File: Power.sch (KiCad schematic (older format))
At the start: 82 parts, among them J3 USB, J4 OTG, Q1 DTA114YKA, SW1 PWRON, SW2 RST, U1 AllWinner-S3(FBGA-234), U3 AXP209(QFN-48), U4 SY8089AAAC, U5 SY6280AAC

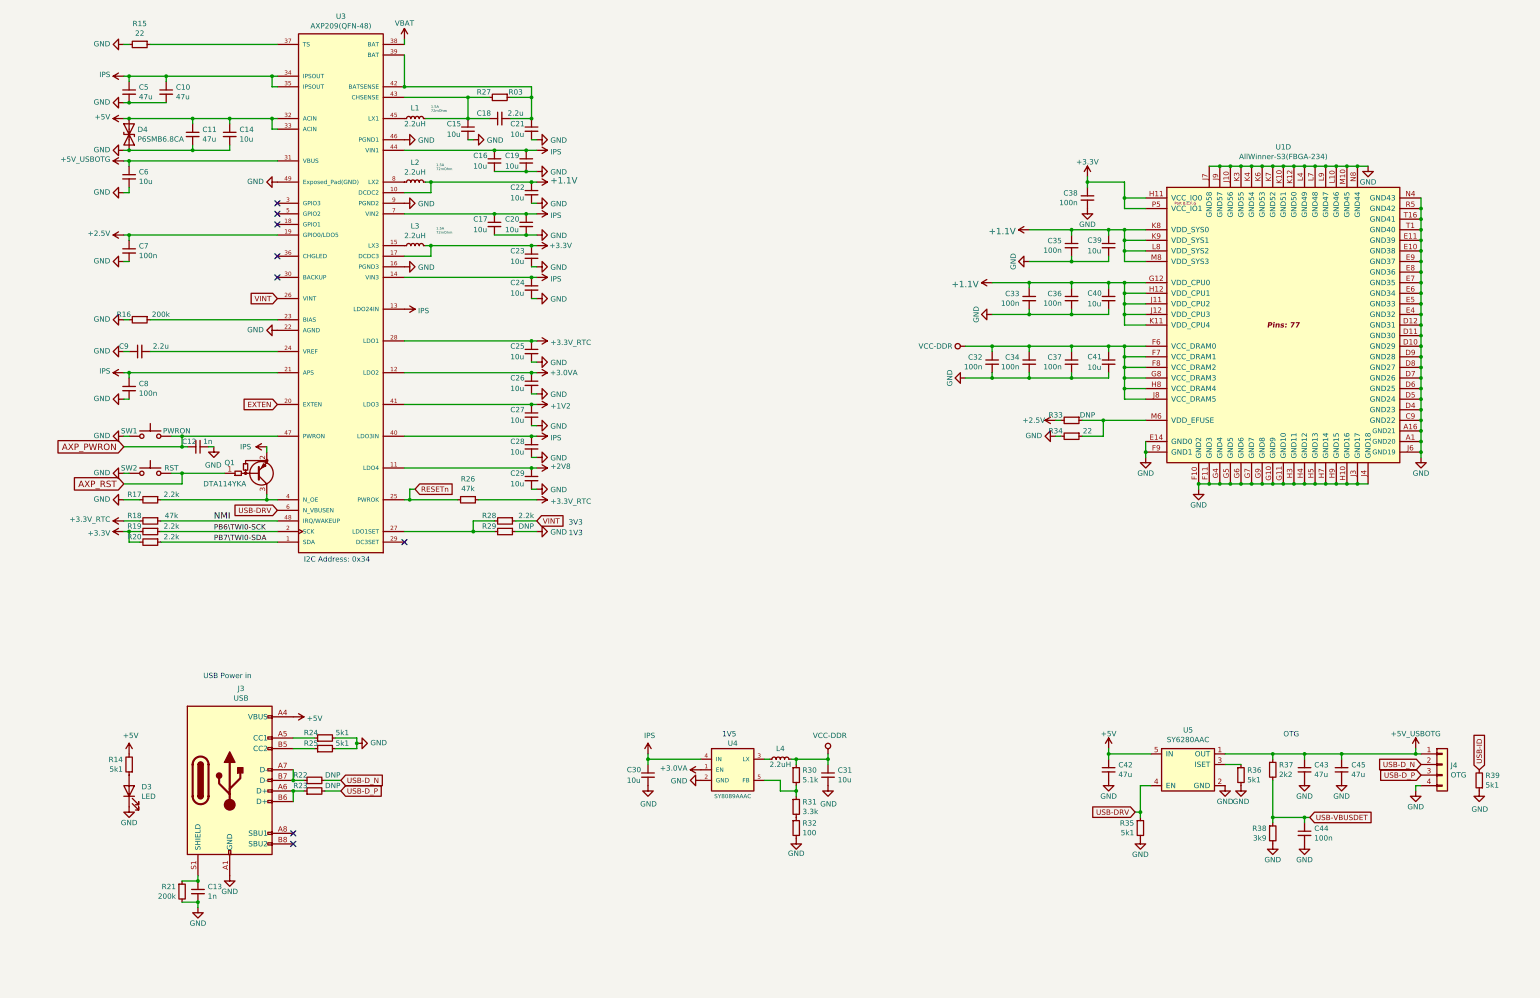
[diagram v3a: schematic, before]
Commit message: update
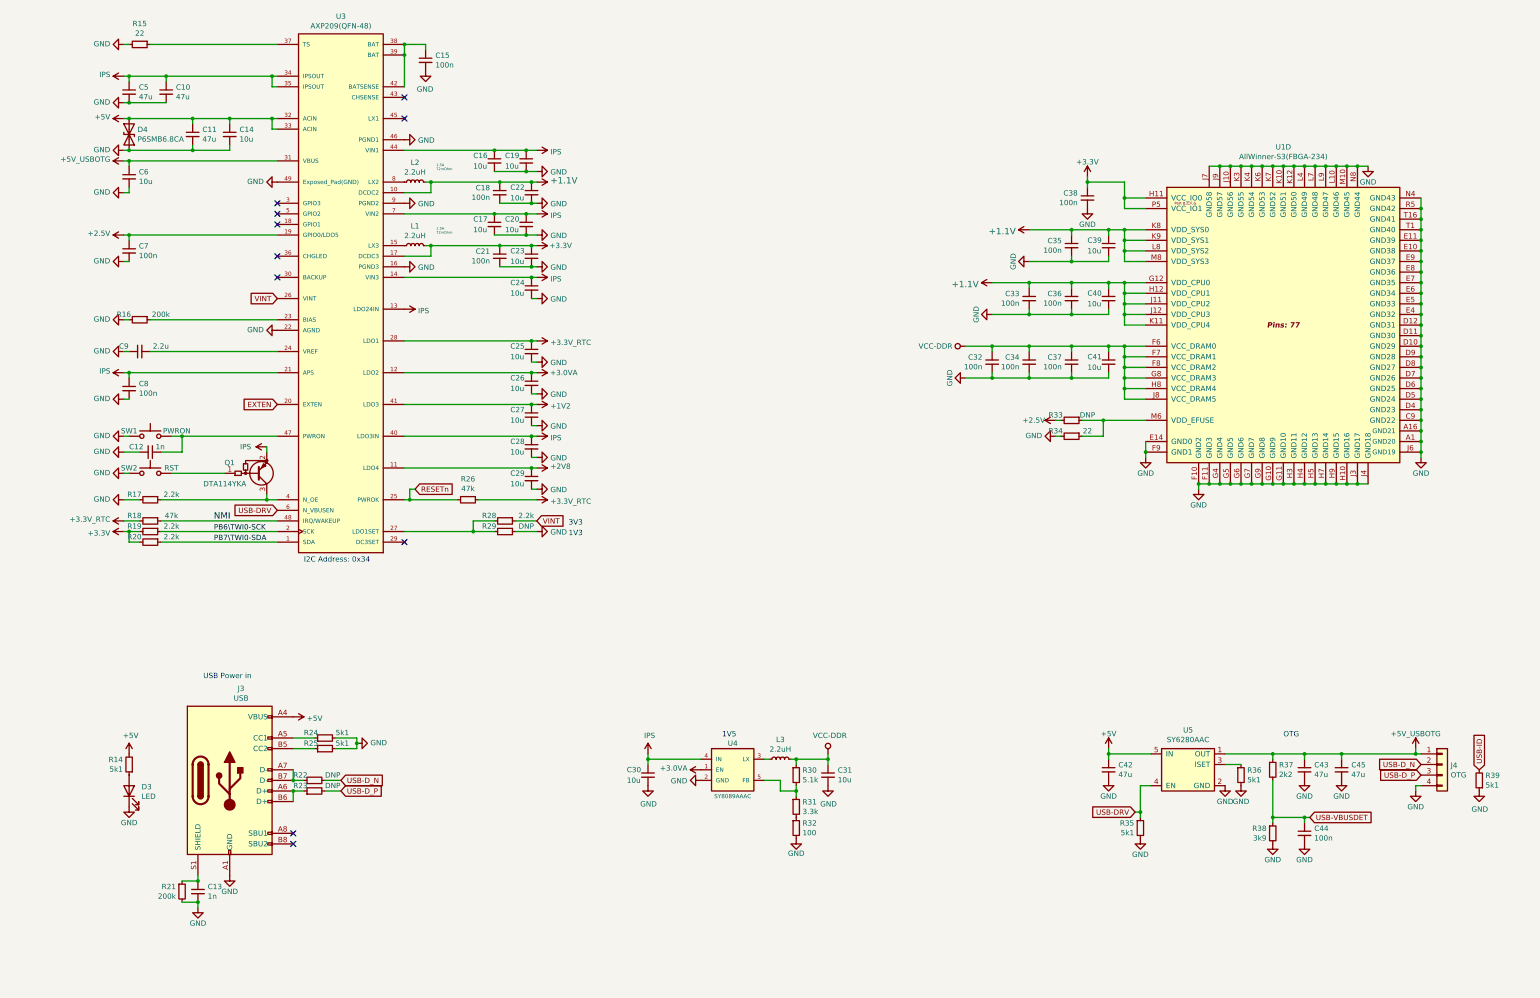
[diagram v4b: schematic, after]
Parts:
- removed L4: 2.2uH, Inductor_SMD:L_Taiyo-Yuden_MD-3030, symbol Device:L_Small
- removed R27: R03, Resistor_SMD:R_1206_3216Metric, symbol Device:R_Small
- C15, C21: value 10u -> 100n; footprint otter:C_0603 -> otter:C_0402
- C18: value 2.2u -> 100n; footprint otter:C_0603 -> otter:C_0402
- D3: footprint otter:LED_0603_1608Metric -> LED_SMD:LED_0603_1608Metric_Castellated
- L1, L2, L3: LCSC (none) -> C167747
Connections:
- net VBAT is gone; now on an unnamed net: U3.38 (BAT)
- net +1.1V: now also C18.1
- net +3V3: now also C21.1, L1.2; no longer L3.2
- net GND: now also C12.2, C18.2; no longer C12.1
- net VCC-DDR: now also L3.2
- net at U4.3 (LX): now also L3.1
- net at U3.15 (LX3): now also L1.1; no longer L3.1
- net at U3.45 (LX1): no longer L1.1
- net at U3.39 (BAT), U3.42 (BATSENSE): now also C15.1; no longer C18.2, C21.1
- net AXP_PWRON: no longer names the net of SW1.2, U3.47 (PWRON)
- net AXP_PWRON: now also C12.1; no longer C12.2
- net AXP_RST: no longer names the net of Q1.1 (B), SW2.2
- now unconnected: U3.43 (CHSENSE)
- no-connect marks 8 -> 10
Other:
- moved on the sheet: C12

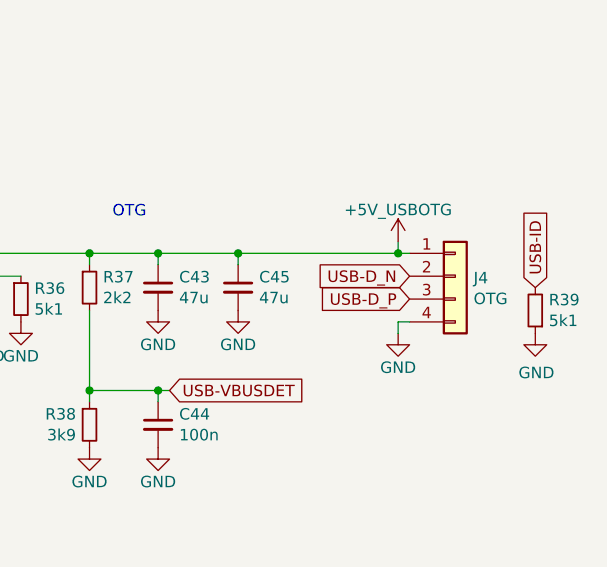
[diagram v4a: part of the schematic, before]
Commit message: update
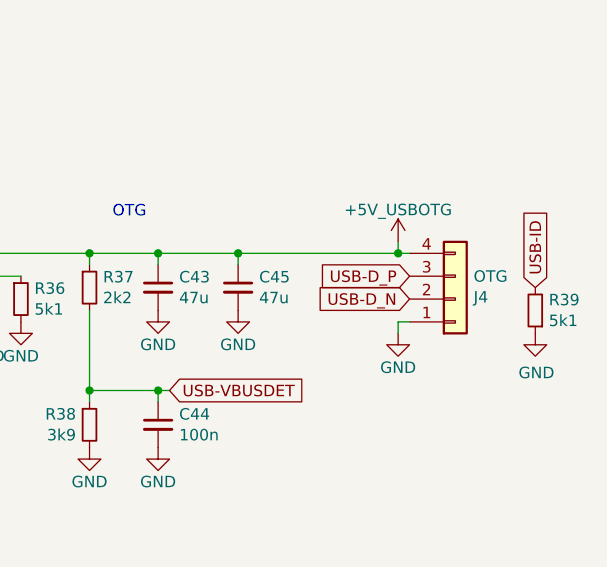
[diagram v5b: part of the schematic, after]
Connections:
- net +5V_USBOTG: now also J4.4 (Pin_4); no longer J4.1 (Pin_1)
- net GND: now also J4.1 (Pin_1); no longer J4.4 (Pin_4)
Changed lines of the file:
@@
 L Connector_Generic:Conn_01x04 J?
 U 1 1 67E47B05
-P 14250 8050
+P 14250 8150
 AR Path="/67E47B05" Ref="J?"  Part="1"
 AR Path="/602ACDF9/67E47B05" Ref="J4"  Part="1"
-F 0 "J4" H 14330 8042 50  0000 L CNN
-F 1 "OTG" H 14330 7951 50  0000 L CNN
-F 2 "Connector_PinHeader_2.00mm:PinHeader_1x04_P2.00mm_Vertical" H 14250 8050 50  0001 C CNN
-F 3 "~" H 14250 8050 50  0001 C CNN
-	1    14250 8050
-	1    0    0    -1
+F 0 "J4" H 14330 8142 50  0000 L CNN
+F 1 "OTG" H 14330 8051 50  0000 L CNN
+F 2 "Connector_PinHeader_2.00mm:PinHeader_1x04_P2.00mm_Vertical" H 14250 8150 50  0001 C CNN
+F 3 "~" H 14250 8150 50  0001 C CNN
+	1    14250 8150
+	1    0    0    1
 $EndComp
 $Comp
@@
 	-1   0    0    1
 $EndComp
+Text GLabel 14050 8150 0    50   Input ~ 0
+USB-D_N
 Text GLabel 14050 8050 0    50   Input ~ 0
-USB-D_N
-Text GLabel 14050 8150 0    50   Input ~ 0
 USB-D_P
 $Comp

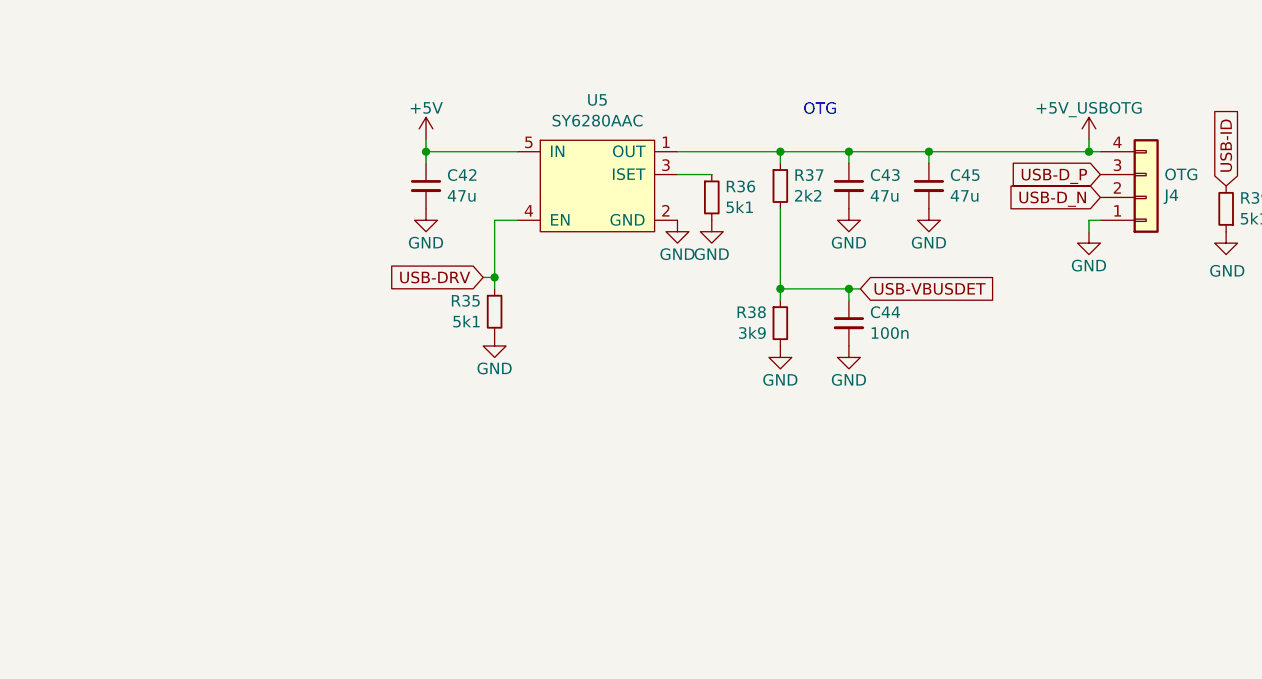
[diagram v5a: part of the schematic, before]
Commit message: update
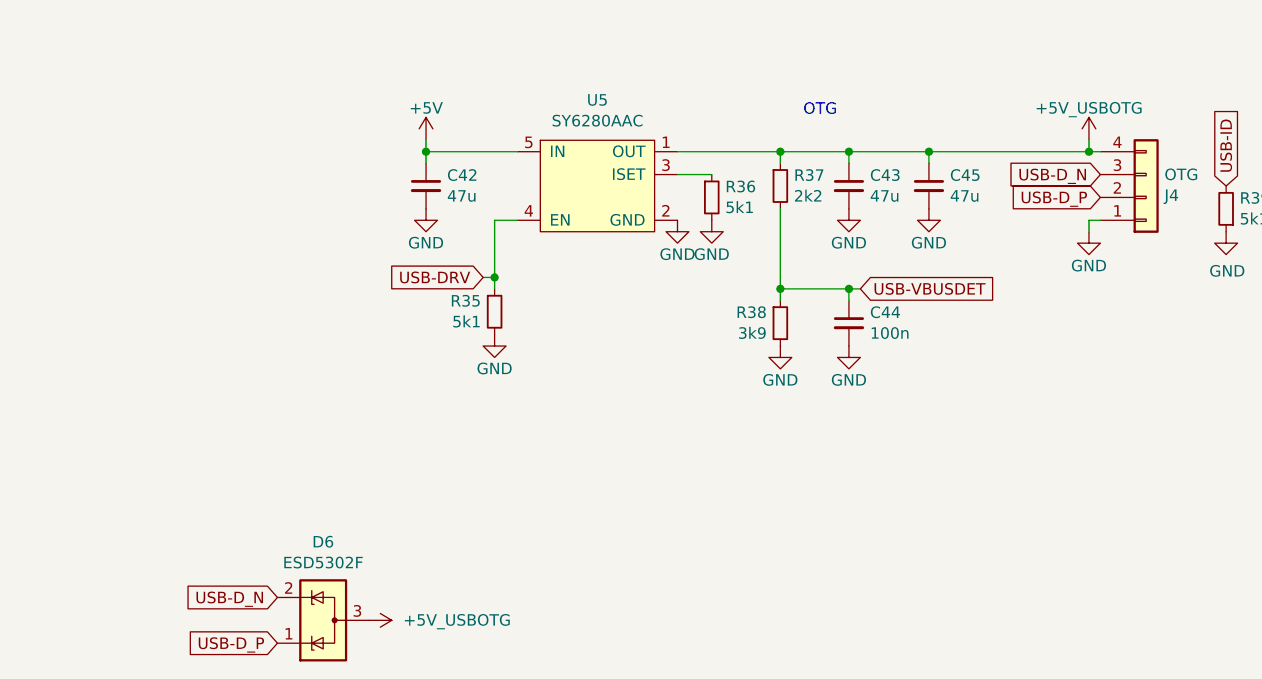
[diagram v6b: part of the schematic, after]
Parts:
- added D6: ESD5302F, Package_TO_SOT_SMD:SOT-23, symbol Power_Protection:SP0502BAHT
- J4: footprint Connector_PinHeader_2.00mm:PinHeader_1x04_P2.00mm_Vertical -> otter:PinHeader_1x04_P2.00mm_Vertical_nosilk_center
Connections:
- net +5V_USBOTG: now also D6.3 (A)
- net USB-D_N: now also J4.3 (Pin_3), D6.2 (K); no longer J4.2 (Pin_2)
- net USB-D_P: now also J4.2 (Pin_2), D6.1 (K); no longer J4.3 (Pin_3)
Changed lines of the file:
@@
 F 0 "J4" H 14330 8142 50  0000 L CNN
 F 1 "OTG" H 14330 8051 50  0000 L CNN
-F 2 "Connector_PinHeader_2.00mm:PinHeader_1x04_P2.00mm_Vertical" H 14250 8150 50  0001 C CNN
+F 2 "otter:PinHeader_1x04_P2.00mm_Vertical_nosilk_center" H 14250 8150 50  0001 C CNN
 F 3 "~" H 14250 8150 50  0001 C CNN
 	1    14250 8150
@@
 	-1   0    0    1
 $EndComp
+Text GLabel 14050 8050 0    50   Input ~ 0
+USB-D_N
 Text GLabel 14050 8150 0    50   Input ~ 0
-USB-D_N
-Text GLabel 14050 8050 0    50   Input ~ 0
 USB-D_P
 $Comp
@@
 Wire Wire Line
 	3500 8300 3400 8300
-Connection ~ 3400 8300
 Wire Wire Line
 	3400 8200 3500 8200
-Connection ~ 3400 8200
 Text Notes 2550 7250 0    50   ~ 0
 USB Power in
@@
 	5350 2550 5650 2550
 Connection ~ 5650 2750
+Text GLabel 10450 9900 0    50   Input ~ 0
+USB-D_N
+Text GLabel 10450 10100 0    50   Input ~ 0
+USB-D_P
+$Comp
+L Power_Protection:SP0502BAHT D6
+U 1 1 5FC7EF96
+P 10650 10000
+F 0 "D6" V 10992 10000 50  0000 C CNN
+F 1 "ESD5302F" V 10901 10000 50  0000 C CNN
+F 2 "Package_TO_SOT_SMD:SOT-23" H 10875 9950 50  0001 L CNN
+F 3 "http://www.littelfuse.com/~/media/files/littelfuse/technical%20resources/documents/data%20sheets/sp05xxba.pdf" H 10775 10125 50  0001 C CNN
+F 4 "C239643" V 10650 10000 50  0001 C CNN "LCSC"
+	1    10650 10000
+	0    -1   -1   0
+$EndComp
+$Comp
+L S3-OLinuXino_Rev_A:+5V_USBOTG #PWR?
+U 1 1 5FC176D0
+P 10850 10000
+AR Path="/5D8A1FAC/5FC176D0" Ref="#PWR?"  Part="1"
+AR Path="/5FC176D0" Ref="#PWR?"  Part="1"
+AR Path="/602ACDF9/5FC176D0" Ref="#PWR0110"  Part="1"
+F 0 "#PWR0110" H 10850 9850 50  0001 C CNN
+F 1 "+5V_USBOTG" V 10850 10150 50  0000 L CNN
+F 2 "" H 10850 10000 60  0000 C CNN
+F 3 "" H 10850 10000 60  0000 C CNN
+	1    10850 10000
+	0    1    1    0
+$EndComp
+Connection ~ 3400 8300
+Connection ~ 3400 8200
 $EndSCHEMATC

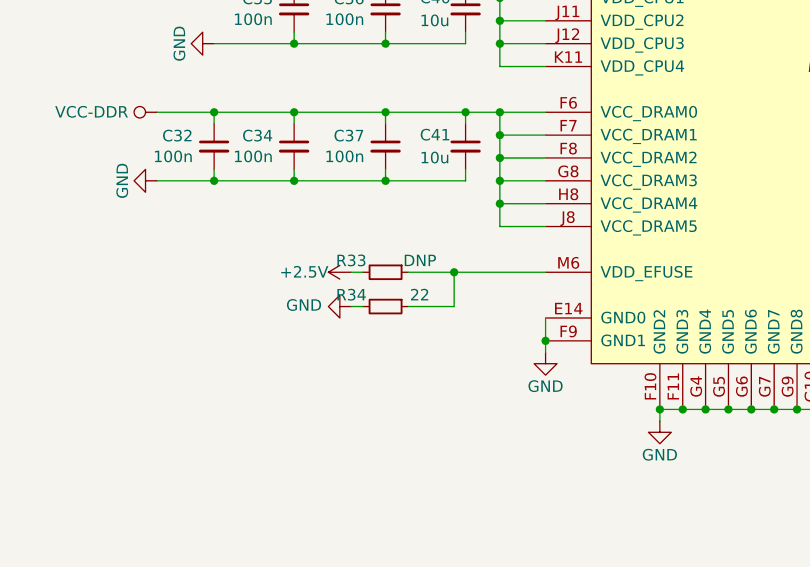
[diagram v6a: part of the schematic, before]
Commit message: update
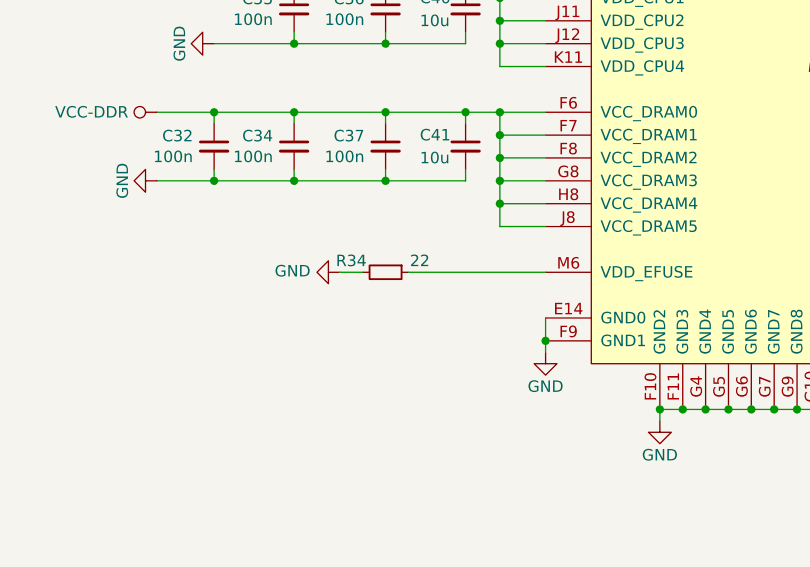
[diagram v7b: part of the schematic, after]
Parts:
- removed R33: DNP, otter:C_0402, symbol Device:R_Small
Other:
- moved on the sheet: R34
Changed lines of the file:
@@
 	0    -1   -1   0
 $EndComp
-Connection ~ 11050 4800
-$Comp
-L S3-OLinuXino_Rev_A:+2.5V #PWR?
-U 1 1 612C27EA
-P 10600 4800
-AR Path="/5D8A1FAC/612C27EA" Ref="#PWR?"  Part="1"
-AR Path="/612C27EA" Ref="#PWR?"  Part="1"
-AR Path="/602ACDF9/612C27EA" Ref="#PWR0134"  Part="1"
-F 0 "#PWR0134" H 10600 4650 50  0001 C CNN
-F 1 "+2.5V" V 10600 4900 50  0000 L CNN
-F 2 "" H 10600 4800 60  0000 C CNN
-F 3 "" H 10600 4800 60  0000 C CNN
-	1    10600 4800
-	0    -1   -1   0
-$EndComp
-Wire Wire Line
-	11050 4800 10850 4800
 Wire Wire Line
 	11250 4500 11250 4400
@@
 Wire Wire Line
 	11250 4600 11250 4500
-Wire Wire Line
-	11050 4800 11450 4800
 $Comp
 L S3-OLinuXino_Rev_A:GND #PWR?
 U 1 1 612C281A
-P 10600 4950
+P 10550 4800
 AR Path="/5D8A1FAC/612C281A" Ref="#PWR?"  Part="1"
 AR Path="/612C281A" Ref="#PWR?"  Part="1"
 AR Path="/602ACDF9/612C281A" Ref="#PWR0135"  Part="1"
-F 0 "#PWR0135" H 10600 4700 50  0001 C CNN
-F 1 "GND" V 10605 4822 50  0000 R CNN
-F 2 "" H 10600 4950 60  0000 C CNN
-F 3 "" H 10600 4950 60  0000 C CNN
-	1    10600 4950
+F 0 "#PWR0135" H 10550 4550 50  0001 C CNN
+F 1 "GND" V 10555 4672 50  0000 R CNN
+F 2 "" H 10550 4800 60  0000 C CNN
+F 3 "" H 10550 4800 60  0000 C CNN
+	1    10550 4800
 	0    1    -1   0
 $EndComp
@@
 $Comp
 L Device:R_Small R?
-U 1 1 6467BD71
+U 1 1 646A8F8C
 P 10750 4800
-AR Path="/6467BD71" Ref="R?"  Part="1"
-AR Path="/602ACDF9/6467BD71" Ref="R33"  Part="1"
-F 0 "R33" V 10700 4650 50  0000 C CNN
-F 1 "DNP" V 10700 4950 50  0000 C CNN
+AR Path="/646A8F8C" Ref="R?"  Part="1"
+AR Path="/602ACDF9/646A8F8C" Ref="R34"  Part="1"
+F 0 "R34" V 10700 4650 50  0000 C CNN
+F 1 "22" V 10700 4950 50  0000 C CNN
 F 2 "otter:C_0402" H 10750 4800 50  0001 C CNN
 F 3 "~" H 10750 4800 50  0001 C CNN
@@
 	0    1    1    0
 $EndComp
-$Comp
-L Device:R_Small R?
-U 1 1 646A8F8C
-P 10750 4950
-AR Path="/646A8F8C" Ref="R?"  Part="1"
-AR Path="/602ACDF9/646A8F8C" Ref="R34"  Part="1"
-F 0 "R34" V 10700 4800 50  0000 C CNN
-F 1 "22" V 10700 5100 50  0000 C CNN
-F 2 "otter:C_0402" H 10750 4950 50  0001 C CNN
-F 3 "~" H 10750 4950 50  0001 C CNN
-	1    10750 4950
-	0    1    1    0
-$EndComp
-Wire Wire Line
-	11050 4800 11050 4950
-Wire Wire Line
-	10850 4950 11050 4950
-Wire Wire Line
-	10600 4800 10650 4800
-Wire Wire Line
-	10600 4950 10650 4950
 $Comp
 L S3-OLinuXino_Rev_A:IPS #PWR?
@@
 Connection ~ 3400 8300
 Connection ~ 3400 8200
+Wire Wire Line
+	10550 4800 10650 4800
+Wire Wire Line
+	10850 4800 11450 4800
 $EndSCHEMATC
